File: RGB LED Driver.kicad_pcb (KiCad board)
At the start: 2 copper layers, 97.1 x 75.7 mm, 106 parts, among them J1 USB_C_Receptacle_USB2.0, J2 Conn_01x06_Pin, Q1 AO3400A, Q2 AO3400A, Q3 AO3400A, Q4 AO3400A, SW1 BOOT, U1 TPS61170DRVR, U10 LM358, U2 AP2112K-3.3TRG1, U3 LM358, U4 USBLC6-2SC6, U5 CP2104-F03-GM, U6 ESP32-WROOM-32, U7 CMXT3904, U8 LM358, U9 LM358

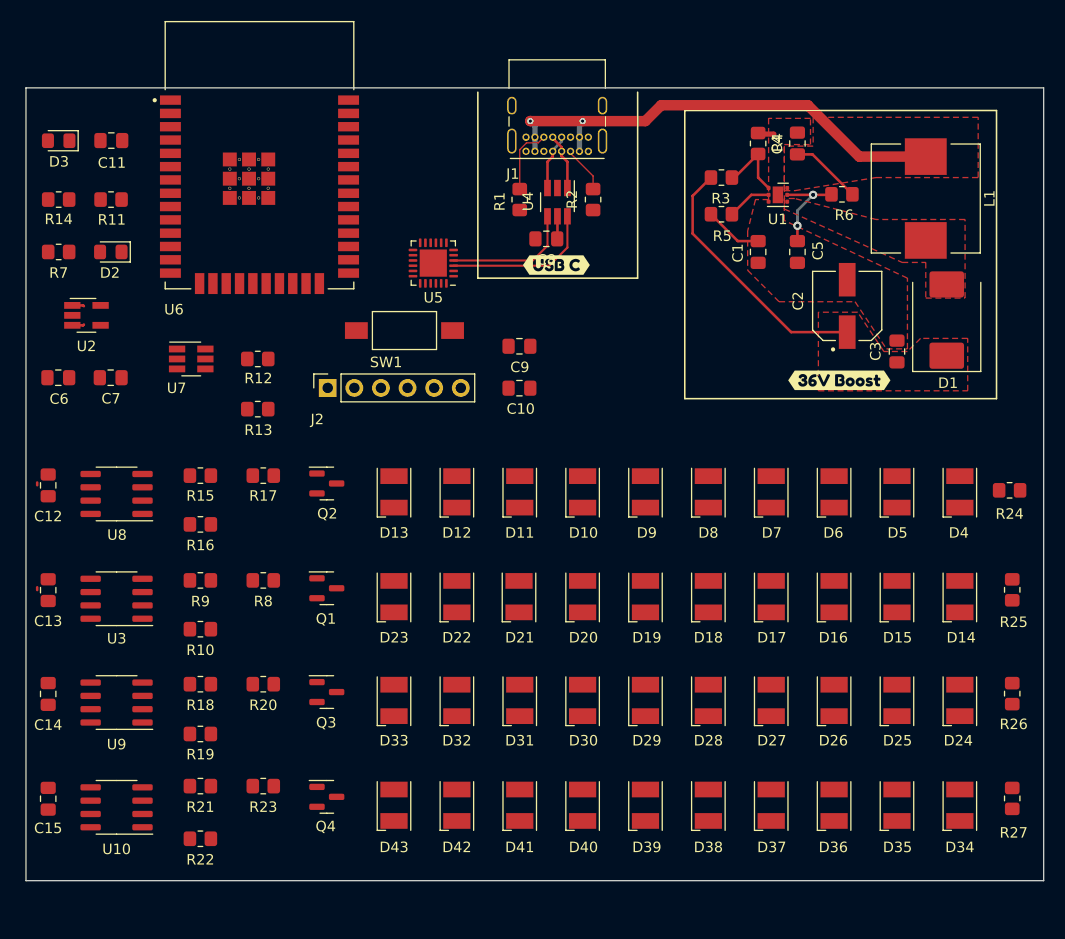
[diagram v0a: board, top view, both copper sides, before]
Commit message: laid out stuff
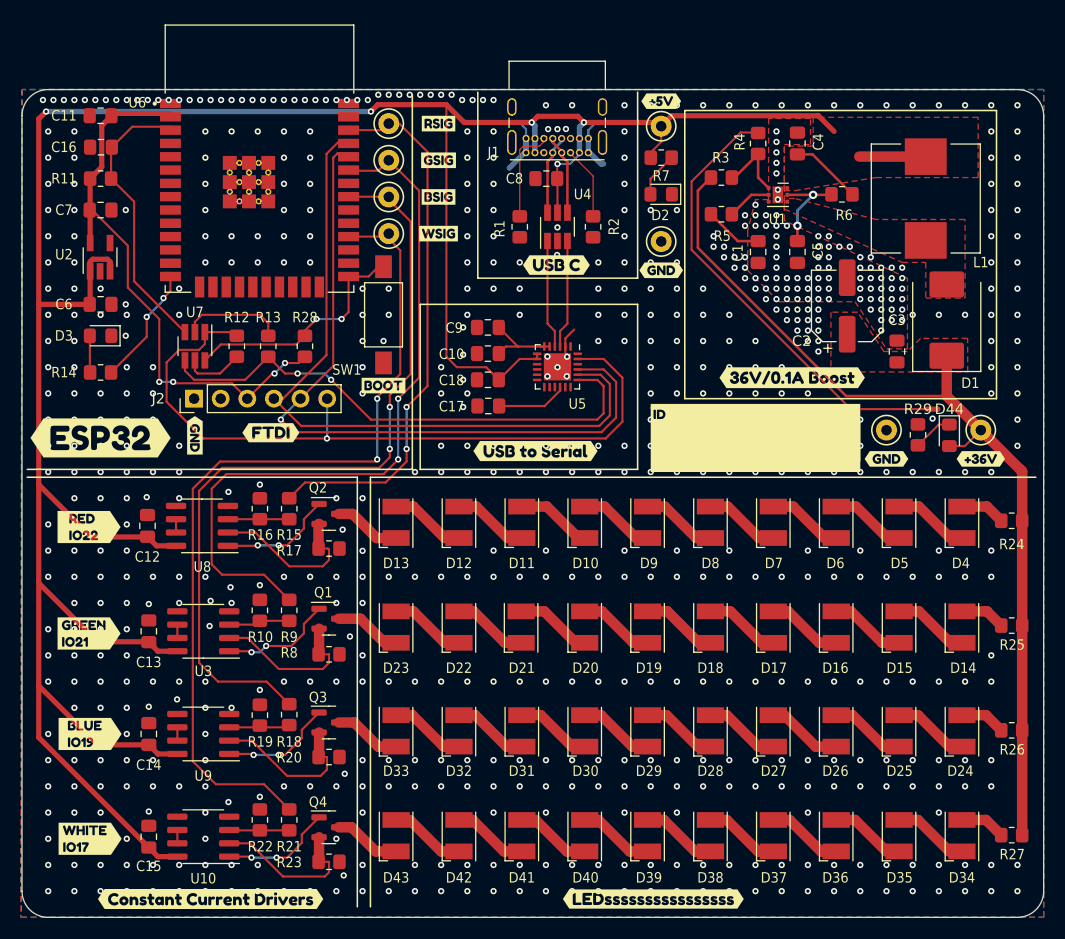
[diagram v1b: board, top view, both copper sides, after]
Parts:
- removed kibuzzard-6592DDAB: G***, kibuzzard-6592DDAB
- added C16: 1uF, Capacitor_SMD:C_0805_2012Metric_Pad1.18x1.45mm_HandSolder, F.Cu at (90.0, 59.0)
- added C17: 1uF, Capacitor_SMD:C_0805_2012Metric_Pad1.18x1.45mm_HandSolder, F.Cu at (127.0, 83.7)
- added C18: 1uF, Capacitor_SMD:C_0805_2012Metric_Pad1.18x1.45mm_HandSolder, F.Cu at (127.0, 81.2)
- added D44: RED LED, LED_SMD:LED_0805_2012Metric_Pad1.15x1.40mm_HandSolder, F.Cu at (171.0, 86.5)
- added R28: 10K, Resistor_SMD:R_0805_2012Metric_Pad1.20x1.40mm_HandSolder, F.Cu at (109.5, 78.0)
- added R29: 300K, Resistor_SMD:R_0805_2012Metric_Pad1.20x1.40mm_HandSolder, F.Cu at (168.0, 86.5)
- added TP1: 5260 (Red), TestPoint:TestPoint_Keystone_5000-5004_Miniature, F.Cu at (143.5, 57.0)
- added TP2: 5264 (Yellow), TestPoint:TestPoint_Keystone_5000-5004_Miniature, F.Cu at (174.0, 86.0)
- added TP3: 5261 (Black), TestPoint:TestPoint_Keystone_5000-5004_Miniature, F.Cu at (143.5, 68.0)
- added TP4: 5261 (Black), TestPoint:TestPoint_Keystone_5000-5004_Miniature, F.Cu at (165.0, 86.0)
- added TP5: 5269 (Purple), TestPoint:TestPoint_Keystone_5000-5004_Miniature, F.Cu at (117.5, 56.8)
- added TP6: 5269 (Purple), TestPoint:TestPoint_Keystone_5000-5004_Miniature, F.Cu at (117.5, 60.2)
- added TP7: 5269 (Purple), TestPoint:TestPoint_Keystone_5000-5004_Miniature, F.Cu at (117.5, 63.8)
- added TP8: 5269 (Purple), TestPoint:TestPoint_Keystone_5000-5004_Miniature, F.Cu at (117.5, 67.2)
- added kibuzzard-65932266: G***, kibuzzard-65932266, F.Cu at (143.5, 54.6)
- added kibuzzard-65932378: G***, kibuzzard-65932378, F.Cu at (165.0, 88.8)
- added kibuzzard-65932378: G***, kibuzzard-65932378, F.Cu at (143.5, 70.8)
- added kibuzzard-6593238E: G***, kibuzzard-6593238E, F.Cu at (174.0, 88.8)
- added kibuzzard-659323CF: G***, kibuzzard-659323CF, F.Cu at (131.5, 88.0)
- added kibuzzard-65932434: G***, kibuzzard-65932434, F.Cu at (106.2, 86.2)
- added kibuzzard-65932443: G***, kibuzzard-65932443, F.Cu at (156.0, 81.0)
- added kibuzzard-65932491: G***, kibuzzard-65932491, F.Cu at (99.0, 86.5)
- added kibuzzard-659324E3: G***, kibuzzard-659324E3, F.Cu at (117.0, 81.8)
- added kibuzzard-65932565: G***, kibuzzard-65932565, F.Cu at (90.0, 86.8)
- added kibuzzard-659325DE: G***, kibuzzard-659325DE, F.Cu at (142.8, 130.8)
- added kibuzzard-65932806: G***, kibuzzard-65932806, F.Cu at (100.5, 130.8)
- added kibuzzard-65932B20: G***, kibuzzard-65932B20, F.Cu at (122.2, 56.8)
- added kibuzzard-65932B45: G***, kibuzzard-65932B45, F.Cu at (122.2, 67.2)
- added kibuzzard-65932B4E: G***, kibuzzard-65932B4E, F.Cu at (122.2, 63.8)
- added kibuzzard-65932B54: G***, kibuzzard-65932B54, F.Cu at (122.2, 60.2)
- added kibuzzard-65932F0E: G***, kibuzzard-65932F0E, F.Cu at (89.0, 125.0)
- added kibuzzard-65932F14: G***, kibuzzard-65932F14, F.Cu at (89.0, 115.0)
- added kibuzzard-65932F1A: G***, kibuzzard-65932F1A, F.Cu at (88.9, 105.4)
- added kibuzzard-65932F21: G***, kibuzzard-65932F21, F.Cu at (88.9, 95.2)
- added kibuzzard-6593379A: G***, kibuzzard-6593379A, F.Cu at (147.5, 84.5)
- C11: value 10uF -> 1uF
- C2: footprint rgb_led_driver_footprints:EEHZA1J100P -> Capacitor_SMD:CP_Elec_6.3x5.8
- J2: footprint Connector_PinSocket_2.54mm:PinSocket_1x06_P2.54mm_Vertical -> Connector_PinHeader_2.54mm:PinHeader_1x06_P2.54mm_Vertical
- moved R7 58.2 mm to (143.5, 60.0)
- moved D2 52.8 mm to (143.5, 63.5)
- moved NT1 30.6 mm to (169.4, 84.0)
- moved D3 19.0 mm to (90.0, 77.0)
- moved R14 17.0 mm to (90.0, 80.5), turned to 180 degrees
- moved C7 16.0 mm to (90.0, 65.0), turned to 0 degrees
- moved U5 15.4 mm to (133.6, 80.0), turned to -90 degrees
- moved J2 12.8 mm to (98.9, 83.0)
- moved C13 10.4 mm to (94.6, 105.2)
- moved C14 10.3 mm to (94.6, 115.0)
- moved C15 10.3 mm to (94.6, 124.8)
- moved C12 10.2 mm to (94.5, 95.1)
- moved R23 9.57 mm to (111.8, 127.2), turned to 0 degrees
- moved R8 9.44 mm to (111.8, 107.4), turned to 0 degrees
- moved R17 9.37 mm to (111.8, 97.3), turned to 0 degrees
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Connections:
- C10 pad 1: +3.3V -> +3V3
- C9 pad 1: +3.3V -> +3V3
- U4 pad 1: Net-(J1-D+-PadA6) -> /USB-Serial/USB_N
- U4 pad 3: Net-(J1-D--PadA7) -> /USB-Serial/USB_P
- U4 pad 4: /USB-Serial/USB_N -> Net-(J1-D+-PadA6)
- U4 pad 6: /USB-Serial/USB_P -> Net-(J1-D--PadA7)
- U5 pad 16: unconnected-(U5-VPP-Pad16) -> Net-(U5-VPP)
- U5 pad 5: +3.3V -> +3V3
- U5 pad 6: +3.3V -> +3V3
- U5 pad 7: +3.3V -> +5V
- U6 pad 27: /ESP32/LED_R -> unconnected-(U6-IO16-Pad27)
- U6 pad 28: /ESP32/LED_G -> /ESP32/LED_W
- U6 pad 30: /ESP32/LED_B -> unconnected-(U6-IO18-Pad30)
- U6 pad 31: /ESP32/LED_W -> /ESP32/LED_B
- U6 pad 33: unconnected-(U6-IO21-Pad33) -> /ESP32/LED_G
- U6 pad 36: unconnected-(U6-IO22-Pad36) -> /ESP32/LED_R
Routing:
- net +5V: track 58.3 -> 280.2 mm, vias 2 -> 5
- net /ESP32/LED_W: track 0.00 -> 82.3 mm, vias 0 -> 2
- net /ESP32/LED_B: track 0.00 -> 76.4 mm, vias 0 -> 2
- net /ESP32/DTR: track 0.00 -> 71.1 mm, vias 0 -> 1
- net /ESP32/LED_G: track 0.00 -> 69.8 mm, vias 0 -> 2
- net /ESP32/TX_CP2102_RX_ESP: track 0.47 -> 69.3 mm, vias 0 -> 1
- net /ESP32/RX_CP2102_TX_ESP: track 0.00 -> 68.6 mm
- net +36V: track 24.7 -> 89.2 mm
- net +3.3V: track 0.00 -> 54.3 mm, vias 0 -> 4
- net /ESP32/LED_R: track 0.00 -> 51.9 mm, vias 0 -> 2
- net /ESP32/RTS: track 0.00 -> 50.2 mm, vias 0 -> 2
- net Net-(NT1-Pad2): track 0.00 -> 43.6 mm
- net /ESP32/RESETn: track 0.00 -> 27.0 mm
- net /ESP32/GPIO0: track 0.00 -> 23.5 mm, vias 0 -> 2
- net GND: track 0.00 -> 15.8 mm, vias 0 -> 701
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- added copper zone on B.Cu, net GND
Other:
- board size 97.1 x 75.7 mm -> 97.5 x 79 mm
- board text added: "RGB LED Light Rev A DG/WS 1/24 MIT PCB Class | pcb.mit.edu github.com/PCB-Design-MIT/ Wi-Fi-Controlled-RGB-Light"
